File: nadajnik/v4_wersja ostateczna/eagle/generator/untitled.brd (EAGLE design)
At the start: 86.3 x 42.9 mm, 26 parts, among them IC1 LM358N, M1 ELECTRET_MICROPHON-F6050AP, T1 BF199

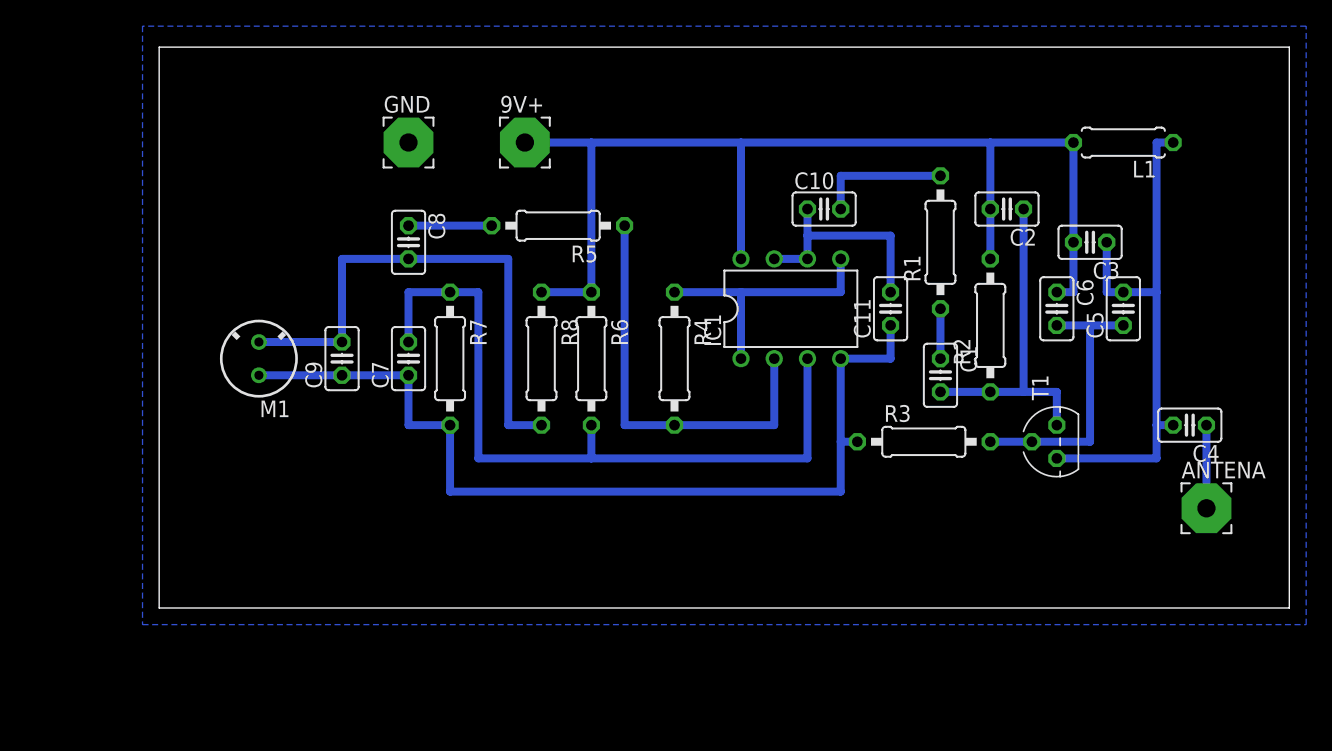
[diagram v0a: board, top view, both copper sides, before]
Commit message: poprawa nadajnika
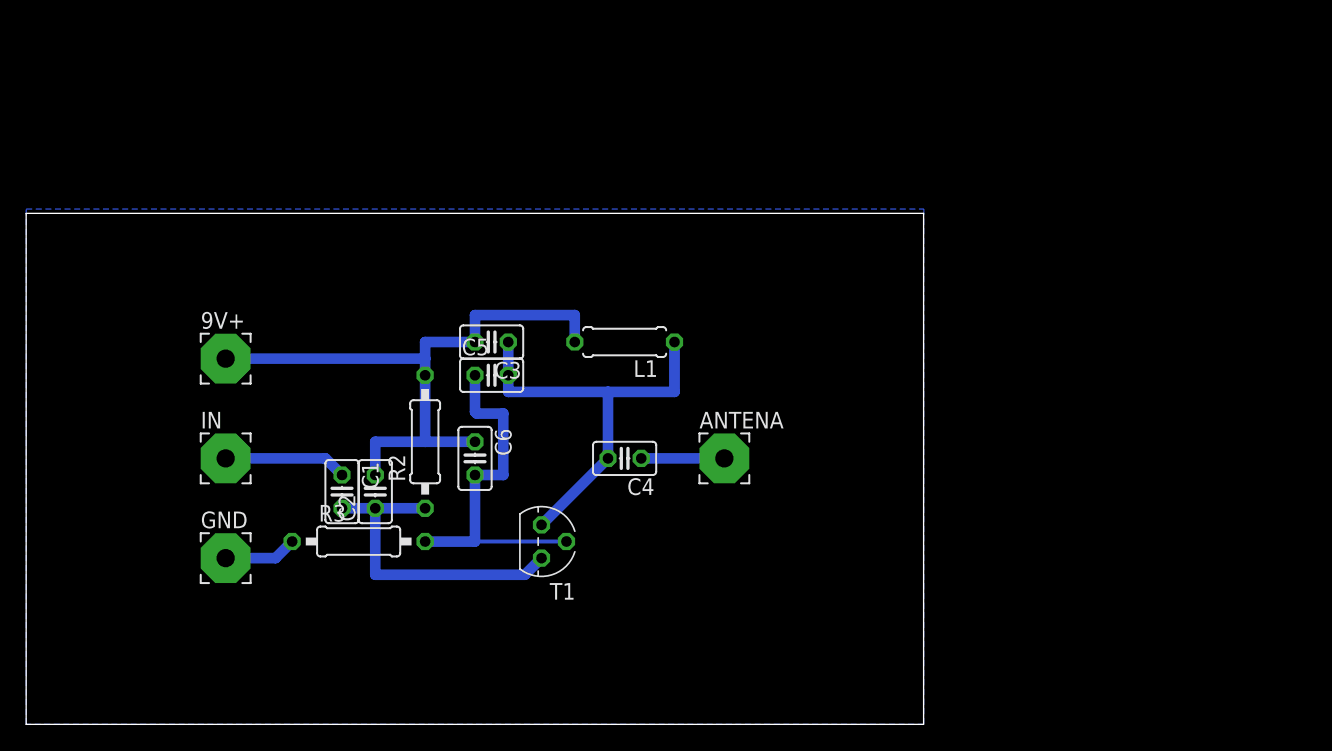
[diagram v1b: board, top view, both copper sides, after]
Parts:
- removed C10: 22u, rcl:C025-025X050
- removed C11, C7, C9: 1n, rcl:C025-025X050
- removed C8: 10u, rcl:C025-025X050
- removed IC1: LM358N, linear:DIL08
- removed M1: ELECTRET_MICROPHON-F6050AP, microphon:F6050AP
- removed R1: 220, rcl:0207/10
- removed R4: 150k, rcl:0207/10
- removed R5: 300, rcl:0207/10
- removed R6: 4.7k, rcl:0207/10
- removed R7: 4.7, rcl:0207/10
- removed R8: 1.8k, rcl:0207/10
- added IN: (no value), wirepad:3,81/1,4
- moved C2 52.9 mm to (16.5, 8.89), turned to 90 degrees
- moved C5 48.5 mm to (25.4, 17.8), turned to 0 degrees
- moved C1 46.6 mm to (14.0, 8.89)
- moved C3 46.4 mm to (25.4, 20.3)
- moved C6 45.9 mm to (24.1, 11.4)
- moved R2 44.1 mm to (20.3, 12.7)
- moved R3 43.8 mm to (15.2, 5.08)
- moved C4 43.3 mm to (35.6, 11.4)
- moved L1 41.0 mm to (35.6, 20.3)
- moved T1 40.1 mm to (29.2, 5.08), turned to 270 degrees
- moved ANTENA 37.0 mm to (43.2, 11.4)
- moved GND 34.7 mm to (5.08, 3.81)
- moved 9V+ 28.2 mm to (5.08, 19.1)
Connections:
- removed net N$10: IC1.2, R4.2, R5.1
- removed net N$11: C7.2, IC1.3, R6.2, R7.1
- removed net N$13: C8.1, R5.2
- removed net N$14: C8.2, C9.2, M1.2, R8.2
- removed net N$2: C1.1, R1.1
- removed net N$4: C10.1, C11.2, IC1.6, IC1.7
- removed net N$9: IC1.1, IC1.5, R4.1
- net GND: no longer C11.1, C7.1, C9.1, IC1.4, M1.1, R7.2
- net N$1: now also C1.1, IN.1; no longer C10.2, R1.2
- net N$7: no longer IC1.8, R6.1, R8.1
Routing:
- net GND: track 71.1 -> 5.61 mm
- net N$11: track 57.1 -> 0.00 mm
- net N$14: track 40.6 -> 0.00 mm
- net N$7: track 87.6 -> 48.6 mm
- net N$10: track 31.8 -> 0.00 mm
- net N$9: track 20.3 -> 0.00 mm
- net N$4: track 17.0 -> 0.00 mm
- net N$6: track 41.9 -> 32.6 mm
- net N$13: track 6.35 -> 0.00 mm
- net N$5: track 21.6 -> 27.7 mm
- net N$2: track 3.81 -> 0.00 mm
- net N$3: track 25.4 -> 24.7 mm
- net N$1: track 10.2 -> 9.42 mm
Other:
- board size 86.3 x 42.9 mm -> 68.6 x 39 mm
